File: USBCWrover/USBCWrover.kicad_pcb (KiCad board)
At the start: 2 copper layers, 31.5 x 40.5 mm, 21 parts, among them J1 USB_C_Receptacle_USB2.0, J2 Conn_02x10_Odd_Even, J3 Conn_02x10_Odd_Even, SW1 SW_Push, U1 UMH3N, U2 CP2104, U3 HX9193-33GB, U4 ESP32-WROVER

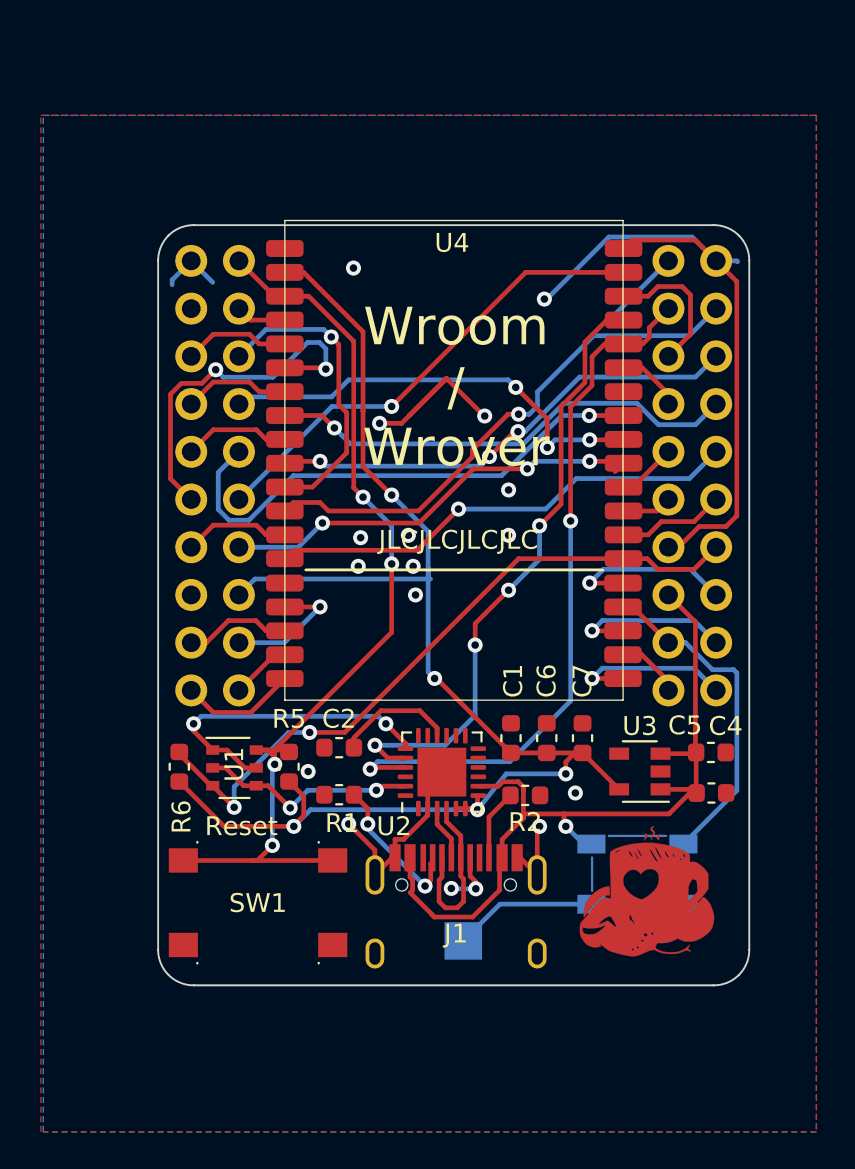
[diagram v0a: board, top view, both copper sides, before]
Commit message: rework
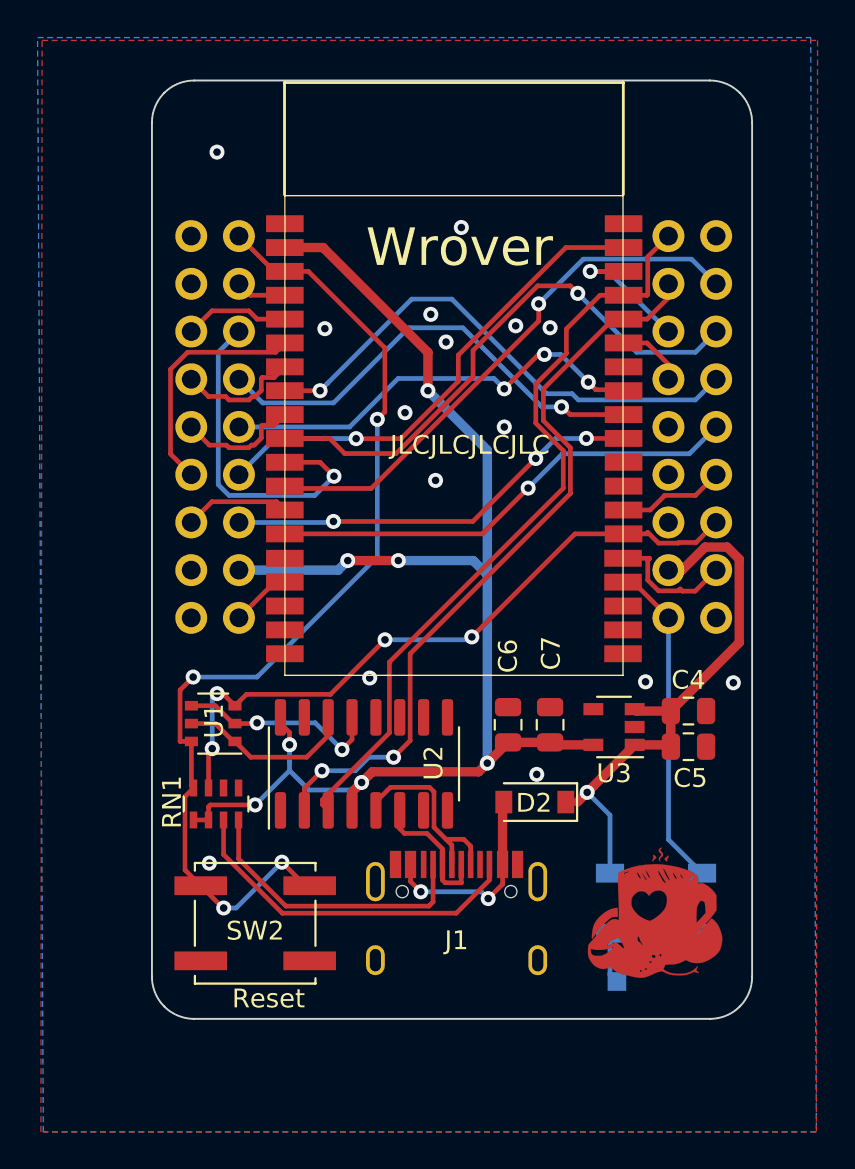
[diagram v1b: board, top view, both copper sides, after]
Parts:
- removed C1: 100nF, Capacitor_SMD:C_0603_1608Metric
- removed C2: 4.7uF, Capacitor_SMD:C_0603_1608Metric
- removed R1, R2: 5.1k, Resistor_SMD:R_0603_1608Metric
- removed R5, R6: 10k, Resistor_SMD:R_0603_1608Metric
- removed SW1: SW_Push, Button_Switch_SMD:SW_Push_1P1T_NO_6x6mm_H9.5mm
- added D2: b5819w, Diode_SMD:D_SOD-123, F.Cu at (145.3, 135.5)
- added RN1: R_Pack04, Resistor_SMD:R_Array_Concave_4x0603, F.Cu at (128.3, 135.6)
- added SW2: SW_Push, Button_Switch_SMD:SW_Push_1P1T_NO_CK_KSC6xxJ, F.Cu at (130.4, 141.9)
- C4, C5, C6, C7: footprint Capacitor_SMD:C_0603_1608Metric -> Capacitor_SMD:C_0805_2012Metric
- J2, J3: footprint Connector_PinHeader_2.54mm:PinHeader_2x10_P2.54mm_Vertical -> Connector_PinHeader_2.54mm:PinHeader_2x09_P2.54mm_Vertical
- TP1: footprint TestPoint:TestPoint_Pad_2.0x2.0mm -> TestPoint:TestPoint_Pad_1.0x1.0mm
- U2: value CP2104 -> CH340C; footprint Package_DFN_QFN:QFN-24-1EP_4x4mm_P0.5mm_EP2.6x2.6mm -> Package_SO:SOIC-16_3.9x9.9mm_P1.27mm
- moved TP1 8.46 mm to (149.7, 145.0)
- moved C4 4.53 mm to (153.5, 130.6)
- moved U2 4.17 mm to (136.2, 133.5)
- moved U3 2.74 mm to (149.5, 131.5)
- moved U1 2.62 mm to (128.2, 131.3), turned to 180 degrees
- moved C6 2.18 mm to (143.9, 131.4)
- moved C7 1.87 mm to (146.1, 131.4)
- moved D1 1.84 mm to (151.7, 140.9)
- moved J2 1.32 mm to (154.9, 105.4)
- moved J3 1.32 mm to (129.5, 105.4)
- moved U4 1.32 mm to (141.0, 103.8)
- moved C5 1.23 mm to (153.5, 132.5)
- moved G*** 1.22 mm to (151.7, 141.5)
- moved J1 0.36 mm to (141.1, 142.8)
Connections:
- J1 pad A4: +5V -> VUSB
- J1 pad A5: Net-(J1-PadA5) -> CC1
- J1 pad A8: Net-(J1-PadA8) -> (no net)
- J1 pad A9: +5V -> VUSB
- J1 pad B4: +5V -> VUSB
- J1 pad B5: Net-(J1-PadB5) -> CC2
- J1 pad B8: Net-(J1-PadB8) -> (no net)
- J1 pad B9: +5V -> VUSB
- J2 pad 10: IO17 -> (no net)
- J2 pad 12: IO16 -> (no net)
- J2 pad 17: SD1_IO8 -> (no net)
- J3 pad 16: Net-(J3-Pad16) -> (no net)
- J3 pad 18: SD2_IO9 -> (no net)
- J3 pad 4: Net-(J3-Pad4) -> (no net)
- U2 pad 1: Net-(U2-Pad1) -> GND
- U2 pad 10: Net-(U2-Pad10) -> (no net)
- U2 pad 11: Net-(U2-Pad11) -> (no net)
- U2 pad 12: Net-(U2-Pad12) -> (no net)
- U2 pad 13: Net-(U2-Pad13) -> SER_DTR
- U2 pad 14: Net-(U2-Pad14) -> SER_RTS
- U2 pad 15: Net-(U2-Pad15) -> (no net)
- U2 pad 16: Net-(C2-Pad1) -> +3V3
- U2 pad 2: GND -> ESP_RXD
- U2 pad 3: USB_D+ -> ESP_TXD
- U2 pad 4: USB_D- -> +3V3
- U2 pad 5: +3V3 -> USB_D+
- U2 pad 6: +3V3 -> USB_D-
- U2 pad 7: +3V3 -> (no net)
- U2 pad 8: +5V -> (no net)
- U2 pad 9: Net-(U2-Pad9) -> (no net)
- U3 pad 4: Net-(U3-Pad4) -> (no net)
- U4 pad 17: SD2_IO9 -> (no net)
- U4 pad 18: SD3_IO10 -> (no net)
- U4 pad 19: CMD_IO11 -> (no net)
- U4 pad 20: CLK_IO6 -> (no net)
- U4 pad 21: SD0_IO7 -> (no net)
- U4 pad 22: SD1_IO8 -> (no net)
- U4 pad 27: IO16 -> (no net)
- U4 pad 28: IO17 -> (no net)
- U4 pad 32: Net-(U4-Pad32) -> (no net)
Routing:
- net GND: track 64.3 -> 0.00 mm
- net CC2: track 0.00 -> 18.8 mm
- net CC1: track 0.00 -> 15.6 mm
- net +5V: track 43.7 -> 30.4 mm
- net VUSB: track 0.00 -> 10.9 mm, vias 0 -> 2
- net SD1_IO8: track 8.96 -> 0.00 mm, vias 1 -> 0
- net CLK_IO6: track 8.96 -> 0.00 mm, vias 1 -> 0
- net Net-(J1-PadA5): track 8.10 -> 0.00 mm, vias 2 -> 0
- net SER_RTS: track 16.9 -> 9.47 mm, vias 2 -> 0
- net IO34: track 19.2 -> 12.7 mm, vias 2 -> 0
- net Net-(C2-Pad1): track 6.35 -> 0.00 mm
- net CMD_IO11: track 6.22 -> 0.00 mm
- net SD2_IO9: track 5.69 -> 0.00 mm
- net Net-(D1-Pad4): track 7.63 -> 2.92 mm
- net USB_D+: track 6.02 -> 10.7 mm, vias 2 -> 0
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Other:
- board size 31.5 x 40.5 mm -> 31.9 x 49.9 mm
- board text added: "GND IO27 IO25 IO32 IO12 IO4 IO0 IO2 NC"
- board text added: "GND NC I 39 I 35 IO33 I 34 IO14 NC NC"
- board text added: "RST I 36 IO26 IO18 IO19 IO23 IO5 3.3v IO13"
- board text added: "TXD RXD IO22 IO21 NC NC GND 5V IO15"
- board text added: "Wrover"
- board text removed: "GND IO27 IO25 IO32 TDI IO4 IO0 IO2 SD1 CLK"
- board text removed: "GND NC SVN IO35 IO33 IO34 TMS NC SD2 CMD"
- board text removed: "RST SVP IO26 IO18 IO19 IO23 IO5 3.3v TCK SD3"
- board text removed: "TXD RXD IO22 IO21 IO17* IO16* GND 5V TDD SD0"
- board text removed: "Wroom / Wrover"
